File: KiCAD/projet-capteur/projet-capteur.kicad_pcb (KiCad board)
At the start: 2 copper layers, 68.6 x 53.3 mm, 24 parts, among them J1 Power, J2 Analog, J3 Digital/PWM, J4 Digital/PWM, U2 LTC1050

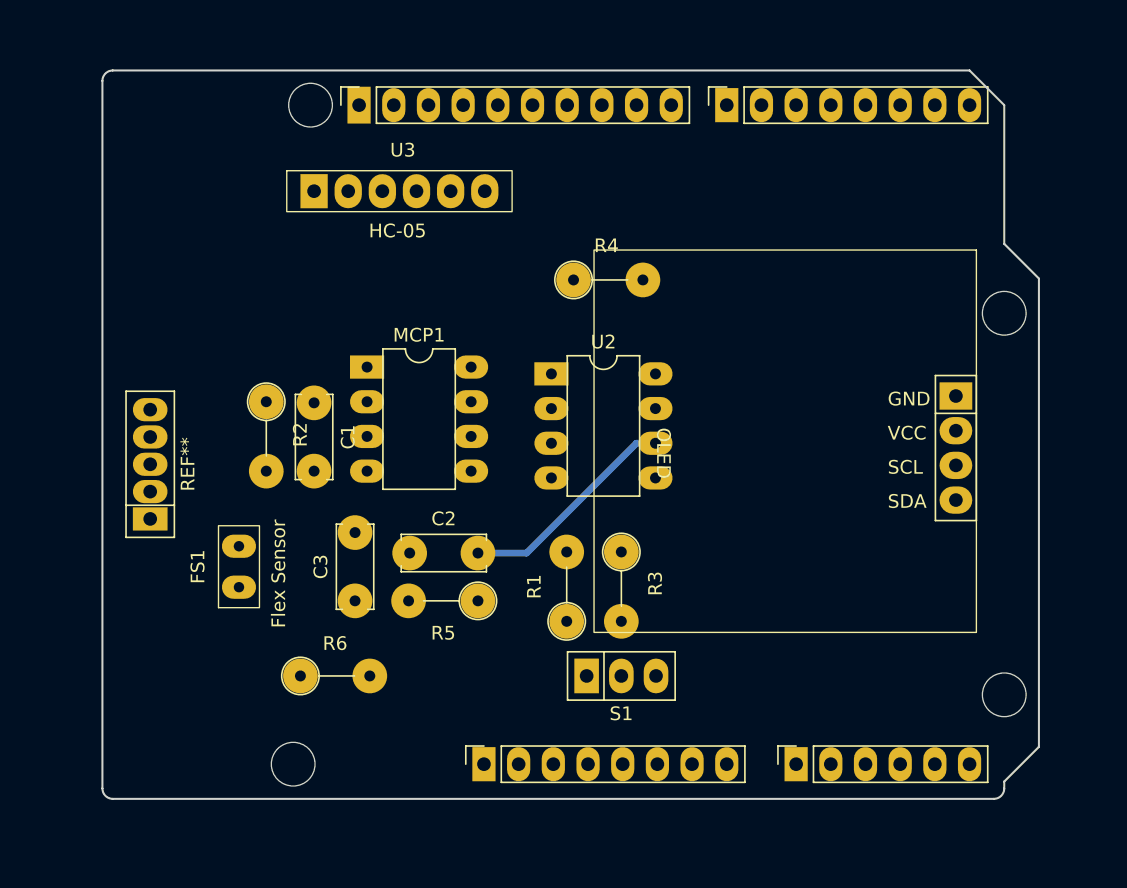
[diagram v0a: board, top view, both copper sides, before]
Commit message: Seance Realisation du shield 12.03 v2
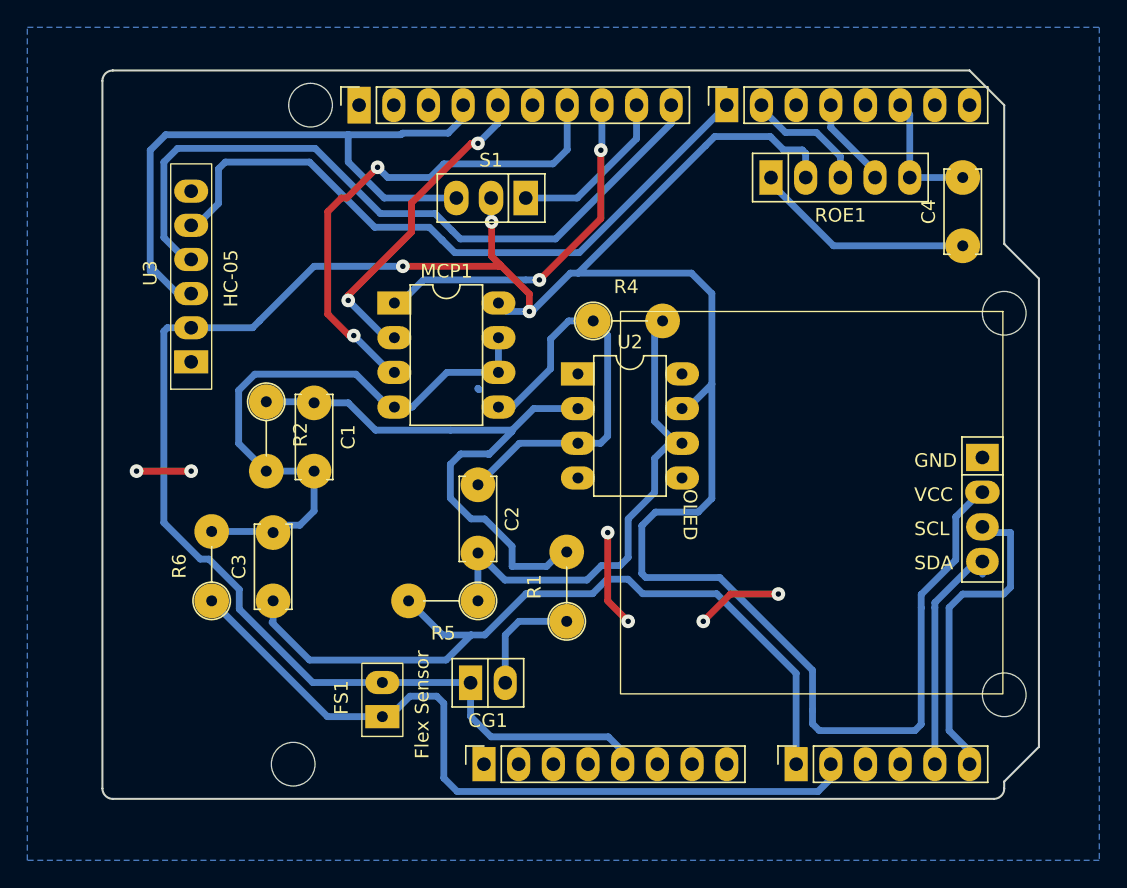
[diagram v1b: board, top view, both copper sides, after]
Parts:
- removed R3: 1k, Resistor_THT:R_Axial_DIN0207_L6.3mm_D2.5mm_P5.08mm_Vertical
- removed REF**: Rotary Encoder, MyLibEmpreinte:Rotary Encoder
- added C4: C, Capacitor_THT:C_Disc_D6.0mm_W2.5mm_P5.00mm, F.Cu at (163.0, 59.5)
- added CG1: ~, MyLibEmpreinte:Capteur Graphene, F.Cu at (128.2, 91.5)
- added ROE1: ~, MyLibEmpreinte:RotaryEncoder, F.Cu at (154.0, 54.5)
- R6: value R -> 10k
- moved S1 36.3 mm to (128.5, 56.0), turned to 180 degrees
- moved U3 16.6 mm to (106.5, 61.5), turned to 90 degrees
- moved FS1 14.2 mm to (120.5, 92.6)
- moved R6 8.51 mm to (108.0, 85.5), turned to 90 degrees
- moved C2 7.07 mm to (127.5, 77.0), turned to -90 degrees
- moved C3 6.00 mm to (112.5, 85.5)
- moved MCP1 5.10 mm to (121.4, 63.7)
- moved U1 4.90 mm to (164.4, 78.8)
- moved R4 3.33 mm to (135.9, 65.0)
- moved U2 1.94 mm to (134.8, 68.9)
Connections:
- C2 pad 1: Net-(U2-+) -> R3
- FS1 pad 1: Net-(FS1-FlexPin) -> Sortie Flex
- J2 pad 2: /A1 -> Sortie Flex
- J3 pad 10: /8 -> TX
- J4 pad 1: /7 -> RX
- J4 pad 2: /*6 -> ROE 3
- J4 pad 4: /4 -> ROE 4
- J4 pad 6: /2 -> ROE 5
- MCP1 pad 5: unconnected-(MCP1-P0A-Pad5) -> R3
- MCP1 pad 6: unconnected-(MCP1-P0W-Pad6) -> GND
- MCP1 pad 7: unconnected-(MCP1-P0B-Pad7) -> GND
- R4 pad 1: Net-(U2-+) -> R3
- R6 pad 1: Net-(FS1-FlexPin) -> Sortie Flex
- U2 pad 3: Net-(U2-+) -> R3
- U3 pad 4: /*3 -> TX
- U3 pad 5: /2 -> RX
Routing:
- net 5V: track 0.00 -> 208.7 mm, vias 0 -> 3
- net GND: track 0.00 -> 128.1 mm, vias 0 -> 6
- net ADC: track 0.00 -> 59.5 mm
- net Sortie Flex: track 0.00 -> 57.0 mm
- net TX: track 0.00 -> 53.4 mm
- net RX: track 0.00 -> 50.0 mm
- net Net-(U2--): track 0.00 -> 44.4 mm
- net /*11: track 0.00 -> 37.4 mm, vias 0 -> 2
- net R3: track 0.00 -> 30.7 mm
- net /*10: track 0.00 -> 26.0 mm, vias 0 -> 2
- net /13: track 0.00 -> 23.6 mm, vias 0 -> 2
- net SCL: track 0.00 -> 23.4 mm
- net Net-(C2-Pad2): track 16.3 -> 36.8 mm
- net SDA: track 0.00 -> 18.2 mm
- net /*9: track 0.00 -> 12.6 mm
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- added copper zone on B.Cu, net GND
